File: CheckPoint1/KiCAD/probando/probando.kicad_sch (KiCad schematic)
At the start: 11 parts, among them J1 Conn_01x02, Q2 BC547, Q3 BC557, Q4 BC557, Q5 BC547, Q6 BC547, Q7 BC547, Q8 BC547, Q9 BC547

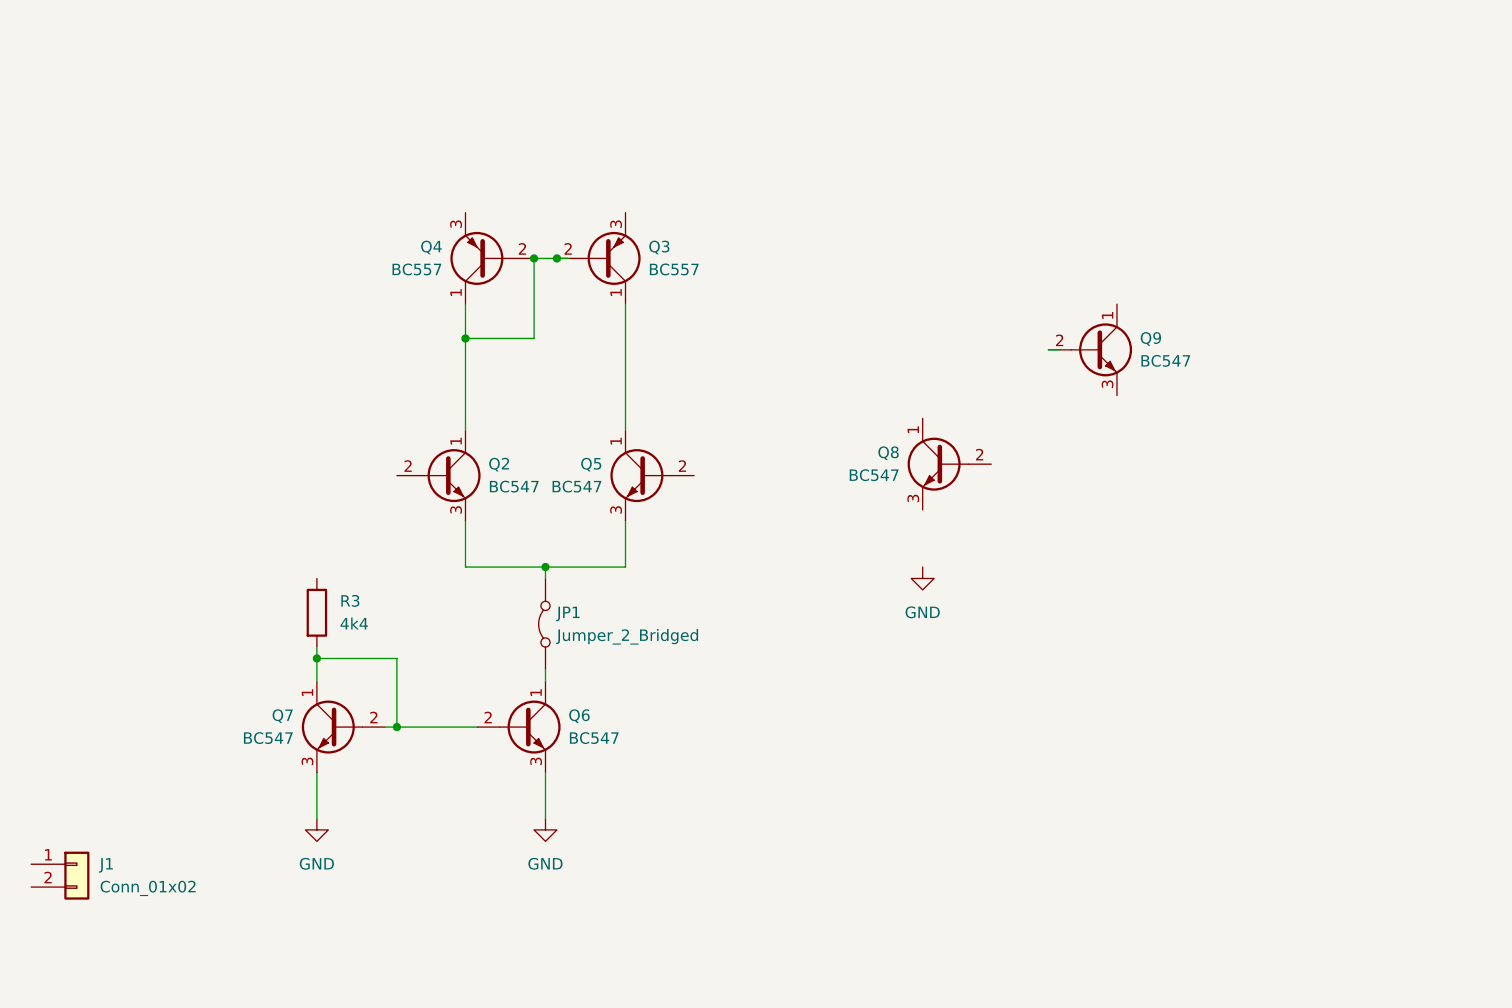
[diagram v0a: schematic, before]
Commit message: hice cositas
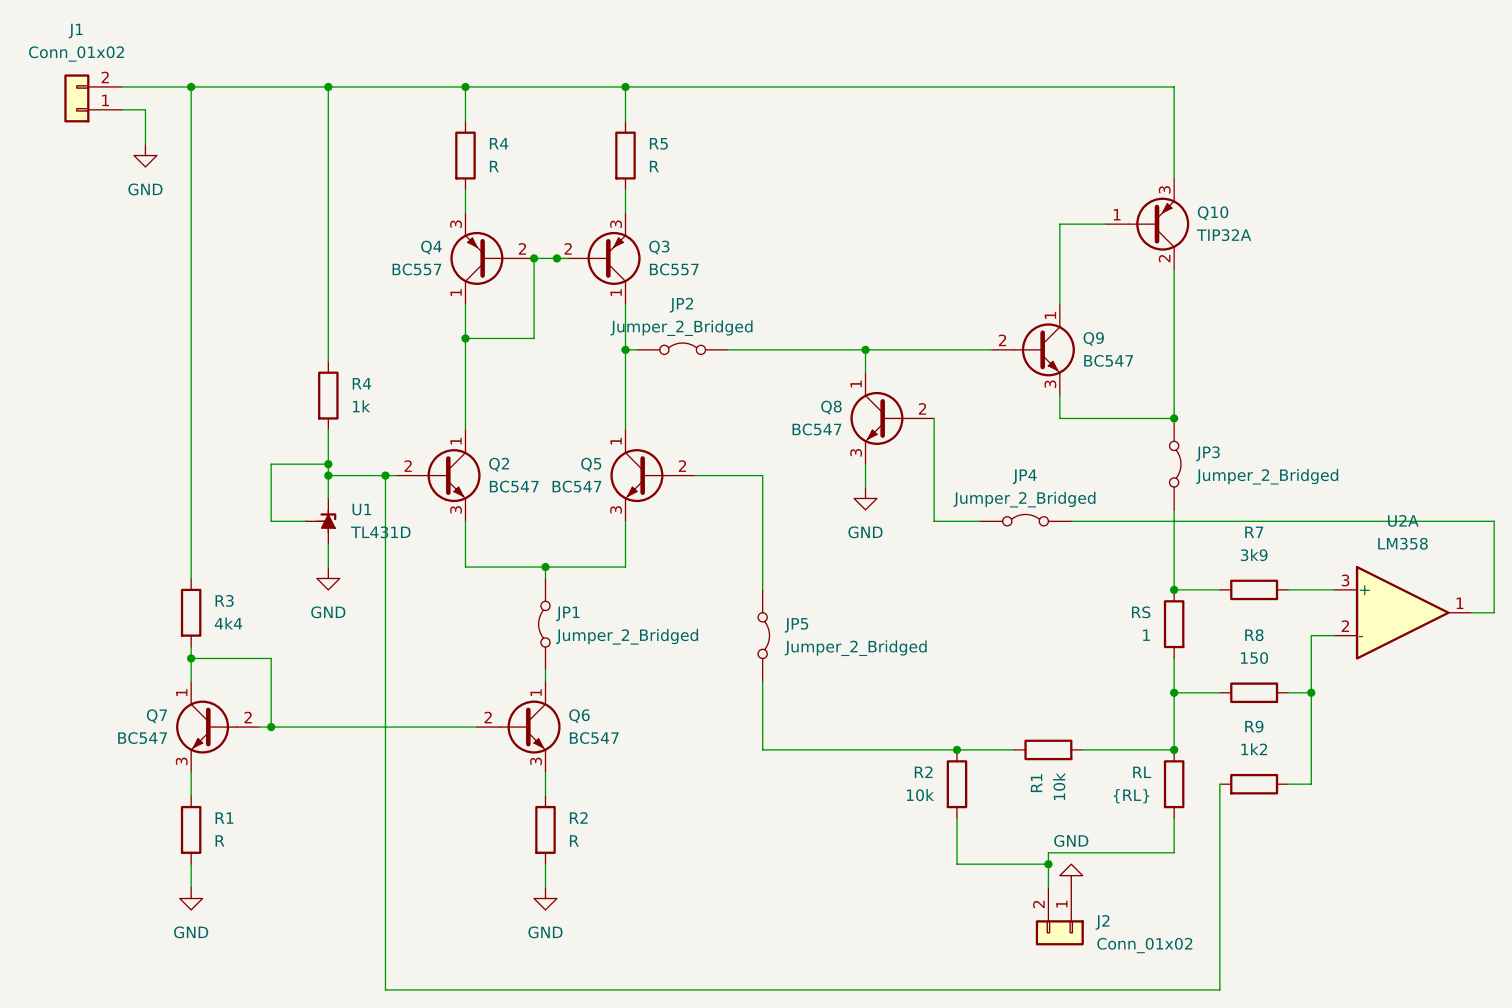
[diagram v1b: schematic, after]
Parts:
- added J2: Conn_01x02, Connector_Samtec_HPM_THT:Samtec_HPM-02-01-x-S_Straight_1x02_Pitch5.08mm, symbol Connector_Generic:Conn_01x02
- added JP2, JP3, JP4, JP5: Jumper_2_Bridged, symbol Jumper:Jumper_2_Bridged
- added Q10: TIP32A, symbol Transistor_BJT:Q_PNP_BCE
- added R1, R2: 10k, symbol Device:R
- added R1, R2, R4, R5: R, symbol Device:R
- added R4: 1k, symbol Device:R
- added R7: 3k9, symbol Device:R
- added R8: 150, symbol Device:R
- added R9: 1k2, symbol Device:R
- added RL: {RL}, symbol Device:R
- added RS: 1, symbol Device:R
- added U1: TL431D, Package_SO:SOIC-8_3.9x4.9mm_P1.27mm, symbol Reference_Voltage:TL431D
- added U2: LM358, symbol Amplifier_Operational:LM358
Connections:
- net GND: now also J1.1 (Pin_1), Q8.3 (E), J2.1 (Pin_1), R1.2, R2.2, U1.2 (A), U1.3 (A), U1.6 (A), U1.7 (A); no longer Q6.3 (E), Q7.3 (E)
- net at Q4.3 (E): now also R4.2
- net at Q3.1 (C), Q5.1 (C): now also JP2.1 (A)
- net at Q3.3 (E): now also R5.2
- net at Q5.2 (B): now also JP5.1 (A)
- net at Q2.2 (B): now also R4.2, R9.2, U1.1 (K), U1.8 (REF)
- net at Q9.1 (C): now also Q10.1 (B)
- net at Q9.2 (B): now also Q8.1 (C), JP2.2 (B)
- net at Q9.3 (E): now also JP3.1 (A), Q10.2 (C)
- net at R3.1: now also J1.2 (Pin_2), Q10.3 (E), R4.1, R4.1, R5.1
- net at Q8.2 (B): now also JP4.1 (A)
- new net: Q6.3 (E), R2.1
- new net: JP4.2 (B), U2.1
- new net: R8.2, R9.1, U2.2 (-)
- new net: R7.2, U2.3 (+)
- new net: R1.2, R8.1, RL.1, RS.2
- new net: J2.2 (Pin_2), R2.2, RL.2
- new net: JP3.2 (B), R7.1, RS.1
- new net: Q7.3 (E), R1.1
- new net: JP5.2 (B), R1.1, R2.1
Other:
- moved on the sheet: J1, Q7, Q8, Q9, R3
